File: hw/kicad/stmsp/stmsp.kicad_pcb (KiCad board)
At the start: 4 copper layers, 42 x 42 mm, 135 parts, among them J1 CONN_02X05, P1 USB_OTG, P2 CONN_01X04, P3 CONN_01X04, P4 CONN_01X02, P5 CONN_01X06, P6 CONN_01X02, Q1 Q_NJFET_GSD, Q2 Q_NJFET_GSD, T1 testpoint, T2 testpoint, T3 testpoint, T4 testpoint, T5 testpoint, U1 USBLC6-4SC6, U10 TLE5012, U2 L6206Q, U3 STM32F303CBTx, U4 USBLC6-4SC6, U5 MCP16331, U6 MIC5504-3.3YM5, U7 TLE5012, U8 SN65176B, U9 SN65176B, Y1 8M

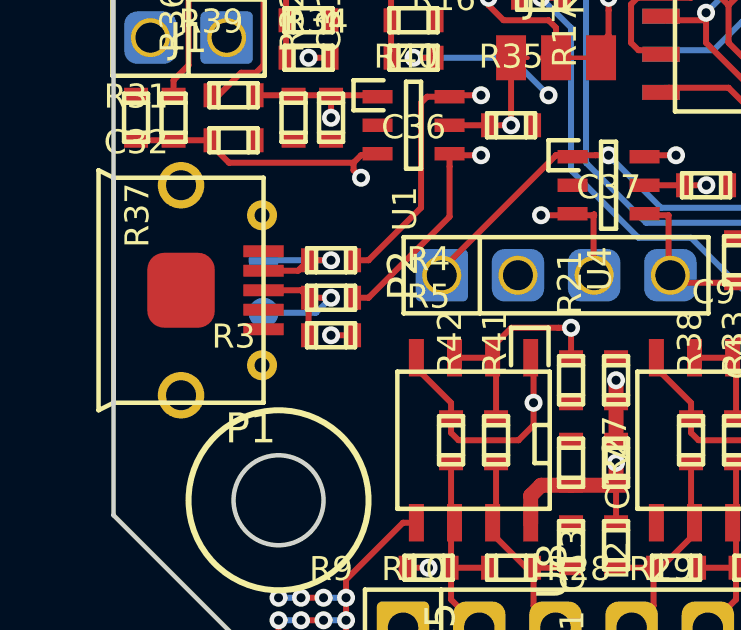
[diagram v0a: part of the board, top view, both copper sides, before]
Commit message: stmsp
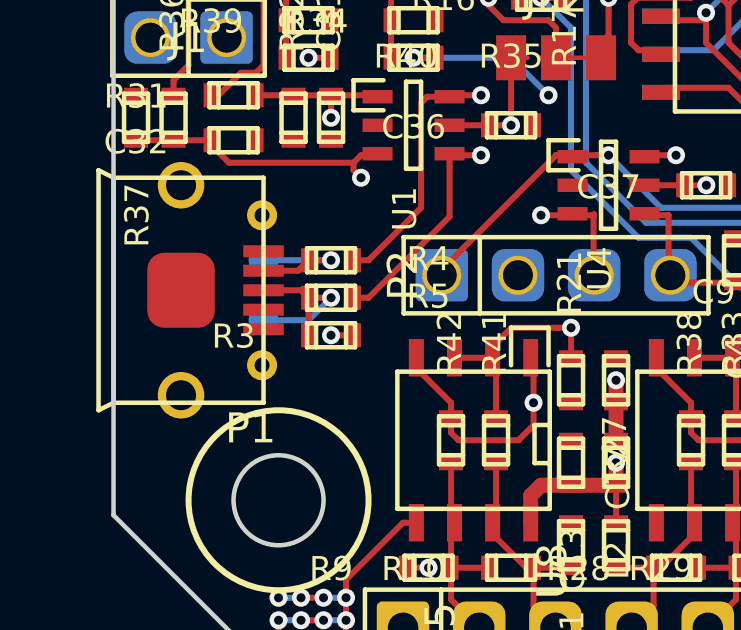
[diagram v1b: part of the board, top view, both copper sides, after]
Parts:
- moved T5 0.25 mm to (55.0, 80.5)
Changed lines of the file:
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@@
     (thickness 1.6)
     (drawings 16)
-    (tracks 1234)
+    (tracks 1235)
     (zones 0)
     (modules 135)
@@
   )
   (module stmbl:Measurement_Point_Round-SMD-Pad_Small (layer B.Cu)
-    (at 55 80.25)
+    (at 55 80.5)
     (descr "Mesurement Point, Round, SMD Pad, DM 1.5mm,")
     (tags "Mesurement Point, Round, SMD Pad, DM 1.5mm,")
@@
   (segment (start 56.5 78.5) (end 56.15 78.85) (width 0.2) (layer F.Cu) (net 4) (status 10))
   (segment (start 56.15 78.85) (end 55 78.85) (width 0.2) (layer F.Cu) (net 4) (status 20))
+  (segment (start 55 80.25) (end 55.25 80.5) (width 0.2) (layer B.Cu) (net 5))
+  (segment (start 55.25 80.5) (end 56.5 80.5) (width 0.2) (layer B.Cu) (net 5))
+  (segment (start 56.5 80.5) (end 57.25 79.75) (width 0.2) (layer B.Cu) (net 5))
   (segment (start 57.25 79.75) (end 56.5 79.75) (width 0.2) (layer F.Cu) (net 5))
-  (segment (start 55 80.25) (end 56.75 80.25) (width 0.2) (layer B.Cu) (net 5))
-  (segment (start 56.75 80.25) (end 57.25 79.75) (width 0.2) (layer B.Cu) (net 5))
   (via (at 57.25 79.75) (size 0.6) (drill 0.3) (layers F.Cu B.Cu) (net 5))
   (segment (start 56.5 81) (end 56.5 79.75) (width 0.2) (layer F.Cu) (net 5) (status 30))

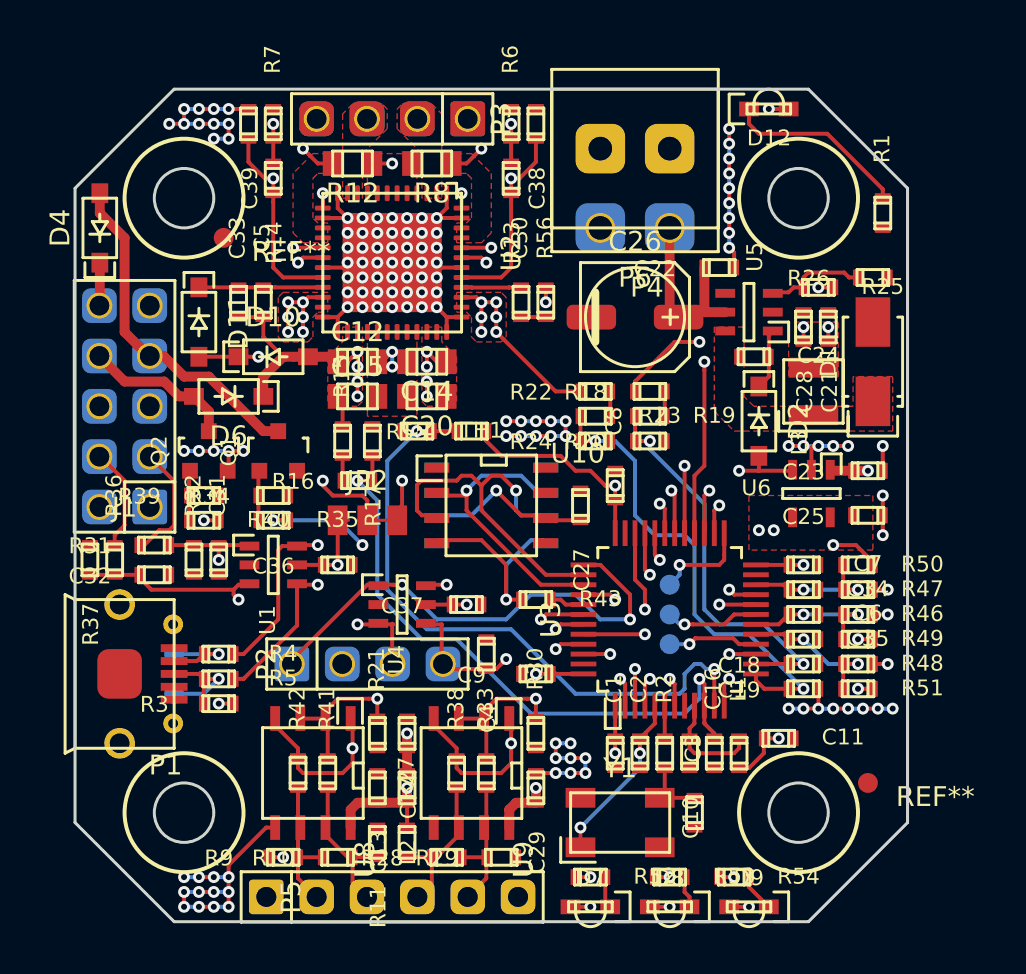
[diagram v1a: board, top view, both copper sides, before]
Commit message: stmsp
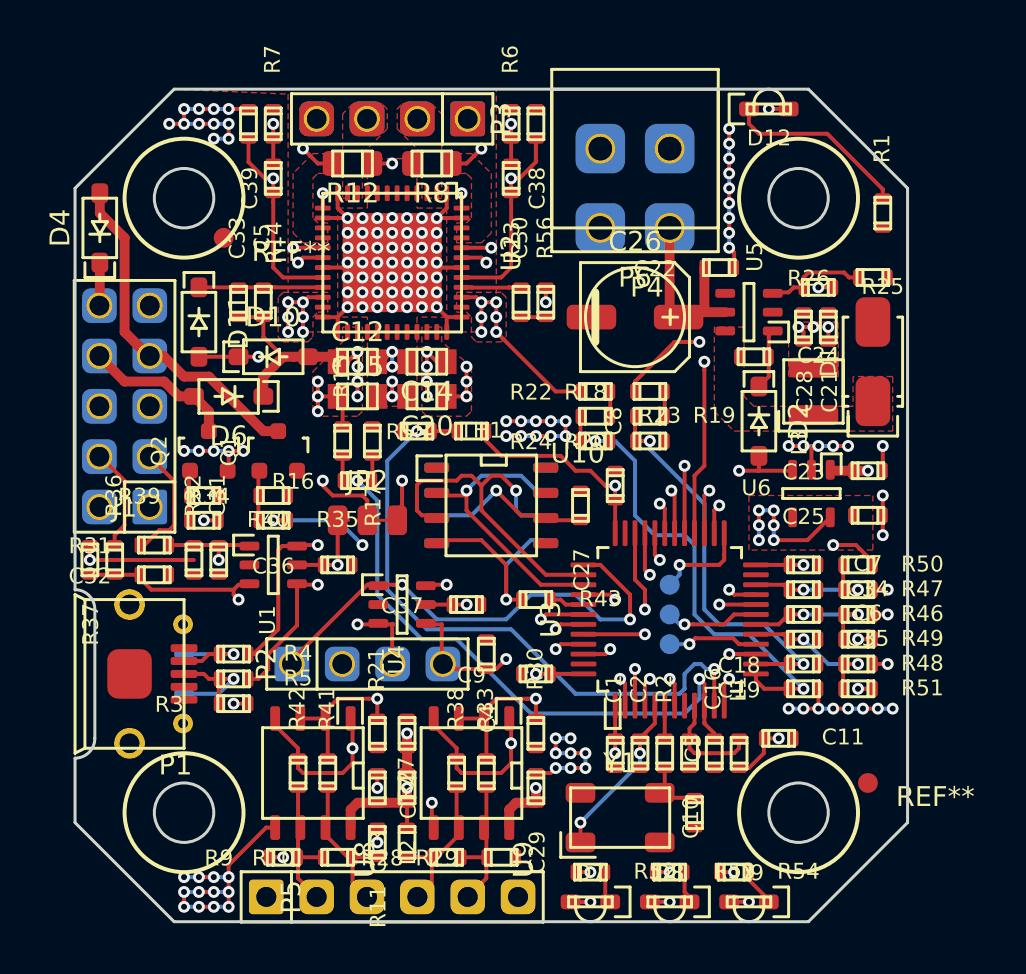
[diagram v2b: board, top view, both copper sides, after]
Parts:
- C26: value 10u -> 22u
- C34, C35, C6: value C -> 18p
- R12, R8: value 0.015 -> 0.02
- R32, R37: value 1k -> 1.5k
- R46, R47, R48: value R -> 3.9k
- R49, R50, R51: value R -> 120
- moved R3 0.75 mm to (58.0, 81.0)
- moved R4 0.75 mm to (58.0, 78.5)
- moved R5 0.75 mm to (58.0, 79.8)
- moved P1 0.50 mm to (52.8, 79.5)
- moved T4 0.50 mm to (55.5, 78.5)
- moved T5 0.50 mm to (55.5, 80.5)
- moved D7 0.25 mm to (76.0, 91.0)
- moved D8 0.25 mm to (80.0, 91.0)
- moved D9 0.25 mm to (84.0, 91.0)
- moved R52 0.25 mm to (76.0, 89.5)
- moved R53 0.25 mm to (80.0, 89.5)
- moved R54 0.25 mm to (83.2, 89.5)
- moved Y1 0.25 mm to (77.5, 86.8)
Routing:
- net +5V: track 106.3 -> 16.4 mm, vias 8 -> 9
- net +3V3: track 109.1 -> 47.6 mm, vias 15 -> 19
- net Net-(C13-Pad1): track 24.0 -> 9.79 mm
- net GND: track 165.5 -> 175.1 mm, vias 125 -> 131
- net VPP: track 43.7 -> 47.5 mm, vias 8 -> 14
- added copper zone on In2.Cu, net +3V3
- added copper zone on In2.Cu, net +5V
- added copper zone on In2.Cu, net Net-(C13-Pad1)
- removed copper zone on In2.Cu, net GND
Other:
- outline, holes or cut-outs redrawn

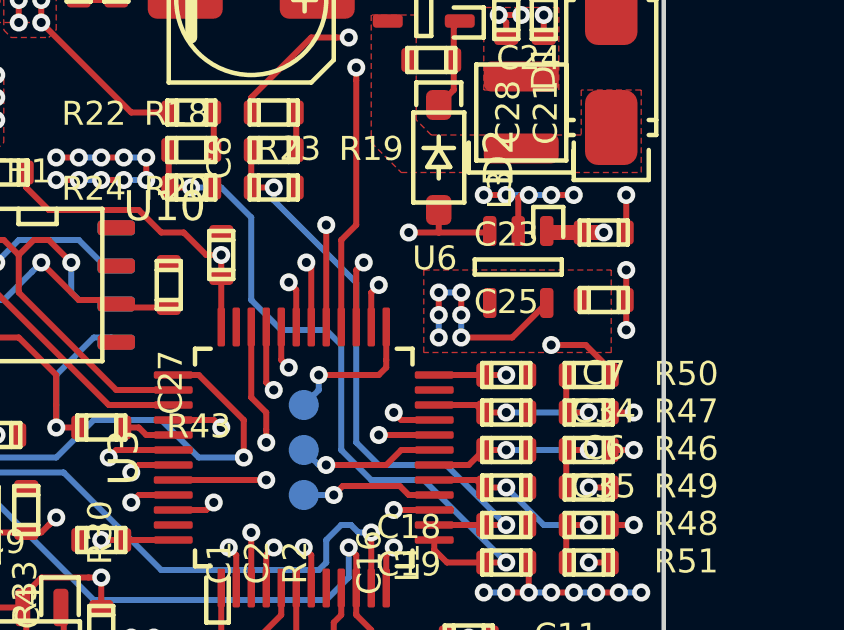
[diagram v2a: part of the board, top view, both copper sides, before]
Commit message: stmsp
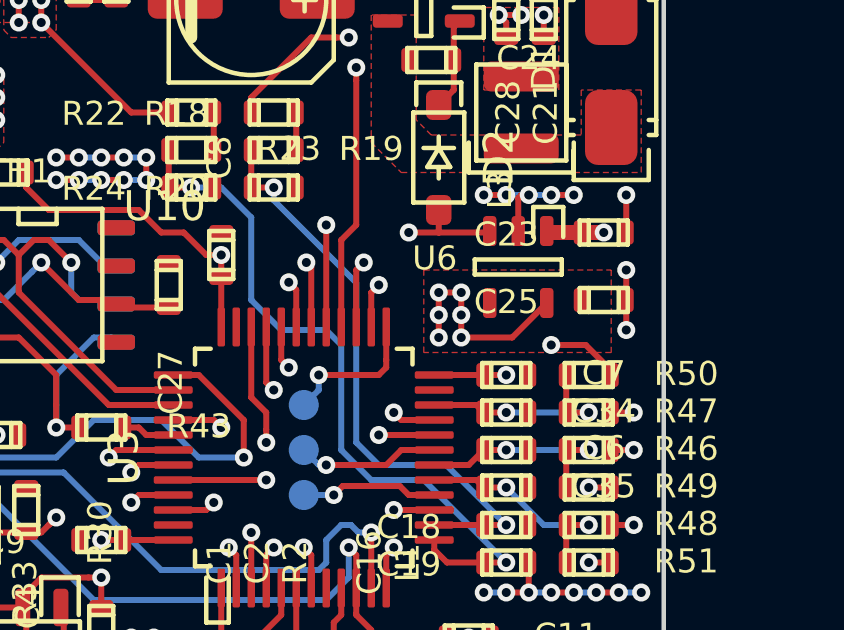
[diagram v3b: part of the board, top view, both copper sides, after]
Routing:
- added copper zone on In2.Cu, net GND
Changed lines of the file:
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@@
   (segment (start 86 74) (end 86.75 74) (width 0.2) (layer F.Cu) (net 77))
   (segment (start 86 74) (end 84.35 74) (width 0.2) (layer F.Cu) (net 77))
-  (segment (start 84.5 72) (end 84.5 72.75) (width 0.2) (layer B.Cu) (net 77))
+  (segment (start 84.5 72) (end 84.5 72.75) (width 0.2) (layer F.Cu) (net 77))
   (via (at 84.5 72.75) (size 0.6) (drill 0.3) (layers F.Cu B.Cu) (net 77))
   (segment (start 84.5 71.25) (end 84.5 72) (width 0.2) (layer F.Cu) (net 77))
   (via (at 84.5 72) (size 0.6) (drill 0.3) (layers F.Cu B.Cu) (net 77))
-  (segment (start 85.25 71.25) (end 84.5 71.25) (width 0.2) (layer B.Cu) (net 77))
+  (segment (start 85.25 71.25) (end 84.5 71.25) (width 0.2) (layer F.Cu) (net 77))
   (via (at 84.5 71.25) (size 0.6) (drill 0.3) (layers F.Cu B.Cu) (net 77))
   (segment (start 85.25 72) (end 85.25 71.25) (width 0.2) (layer F.Cu) (net 77))
   (via (at 85.25 71.25) (size 0.6) (drill 0.3) (layers F.Cu B.Cu) (net 77))
-  (segment (start 85.25 72.75) (end 85.25 72) (width 0.2) (layer B.Cu) (net 77))
+  (segment (start 85.25 72.75) (end 85.25 72) (width 0.2) (layer F.Cu) (net 77))
   (via (at 85.25 72) (size 0.6) (drill 0.3) (layers F.Cu B.Cu) (net 77))
   (segment (start 88.1 71.6) (end 86.95 72.75) (width 0.2) (layer F.Cu) (net 77))
@@
     )
   )
-  (zone (net 0) (net_name "") (layer In1.Cu) (hatch edge 0.508)
-    (connect_pads yes (clearance 0.2))
-    (min_thickness 0.2)
-    (keepout (tracks not_allowed) (vias not_allowed) (copperpour not_allowed))
-    (fill yes (arc_segments 16) (thermal_gap 0.2) (thermal_bridge_width 0.25))
-    (polygon
-      (pts
-        (xy 85.75 66)
-      )
-    )
-  )
   (zone (net 10) (net_name +5V) (layer F.Cu) (hatch edge 0.508)
     (priority 1)
@@
       )
     )
+  )
+  (zone (net 7) (net_name GND) (layer In1.Cu) (hatch edge 0.508)
+    (connect_pads yes (clearance 0.25))
+    (min_thickness 0.25)
+    (fill yes (arc_segments 16) (thermal_gap 0.508) (thermal_bridge_width 0.508))
+    (polygon
+      (pts
+        (xy 63 55.75) (xy 69 55.75) (xy 69 61.75) (xy 63 61.75)
+      )
+    )
+  )
+  (zone (net 7) (net_name GND) (layer In2.Cu) (hatch edge 0.508)
+    (connect_pads yes (clearance 0.25))
+    (min_thickness 0.25)
+    (fill yes (arc_segments 16) (thermal_gap 0.508) (thermal_bridge_width 0.508))
+    (polygon
+      (pts
+        (xy 63.25 50) (xy 68.75 50) (xy 68.75 61.75) (xy 63.25 61.75)
+      )
+    )
+  )
+  (zone (net 0) (net_name "") (layer In2.Cu) (hatch edge 0.508)
+    (connect_pads yes (clearance 0.25))
+    (min_thickness 0.25)
+    (keepout (tracks allowed) (vias allowed) (copperpour not_allowed))
+    (fill yes (arc_segments 16) (thermal_gap 0.508) (thermal_bridge_width 0.508))
+    (polygon
+      (pts
+        (xy 65.75 53.25) (xy 65.5 53.5) (xy 65.5 54) (xy 65.75 54.25) (xy 66.25 54.25)
+        (xy 66.5 54) (xy 66.5 53.5) (xy 66.25 53.25)
+      )
+    )
+  )
+  (zone (net 0) (net_name "") (layer B.Cu) (hatch edge 0.508)
+    (connect_pads yes (clearance 0.25))
+    (min_thickness 0.25)
+    (keepout (tracks allowed) (vias allowed) (copperpour not_allowed))
+    (fill yes (arc_segments 16) (thermal_gap 0.508) (thermal_bridge_width 0.508))
+    (polygon
+      (pts
+        (xy 65.75 53.25) (xy 65.5 53.5) (xy 65.5 54) (xy 65.75 54.25) (xy 66.25 54.25)
+        (xy 66.5 54) (xy 66.5 53.5) (xy 66.25 53.25)
+      )
+    )

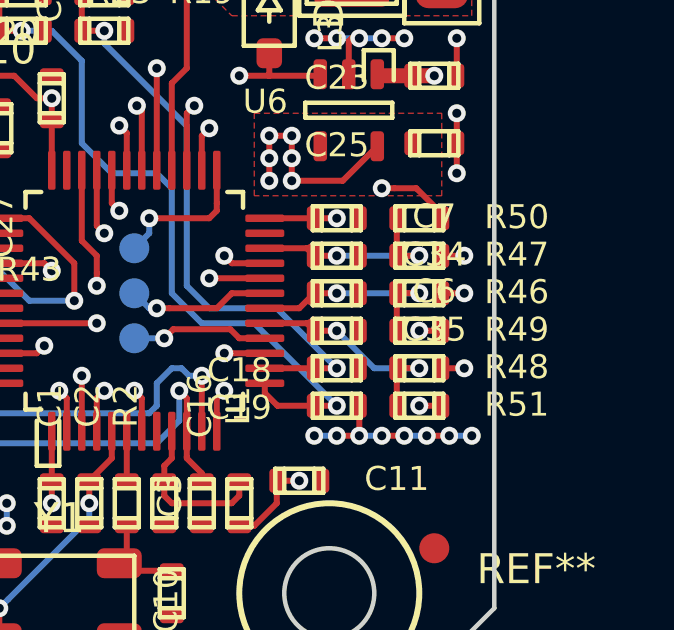
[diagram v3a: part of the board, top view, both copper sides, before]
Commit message: stmsp
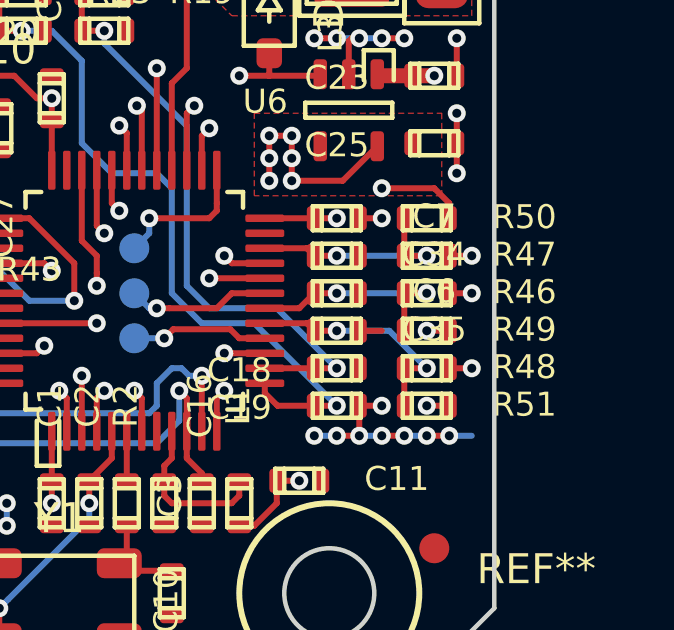
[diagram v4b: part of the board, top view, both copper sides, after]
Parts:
- moved R46 0.25 mm to (89.8, 76.5)
- moved R47 0.25 mm to (89.8, 75.2)
- moved R48 0.25 mm to (89.8, 79.0)
- moved R49 0.25 mm to (89.8, 77.8)
- moved R50 0.25 mm to (89.8, 74.0)
- moved R51 0.25 mm to (89.8, 80.2)
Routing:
- net GND: track 175.1 -> 177.3 mm, vias 131 -> 132
- net Net-(R12-Pad2): track 41.9 -> 42.5 mm
